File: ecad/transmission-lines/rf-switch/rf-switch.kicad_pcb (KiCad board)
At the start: 2 copper layers, 22.9 x 34.3 mm, 5 parts, among them J1 USB_C_Receptacle_USB2.0, J2 Conn_01x05_Pin, SW1 SW_DIP_x01, U1 ADG918BRM, U2 AP7384-33Y

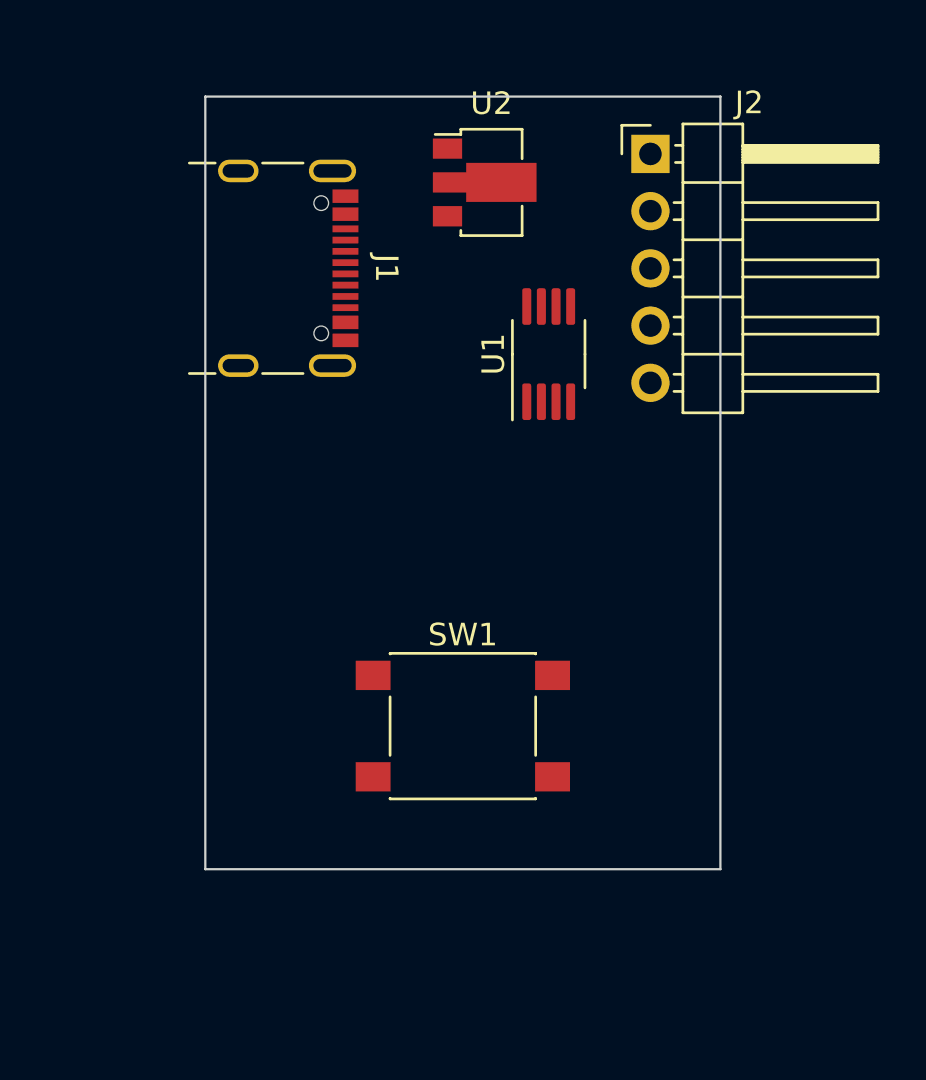
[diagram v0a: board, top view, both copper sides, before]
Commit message: rf-switch: Update
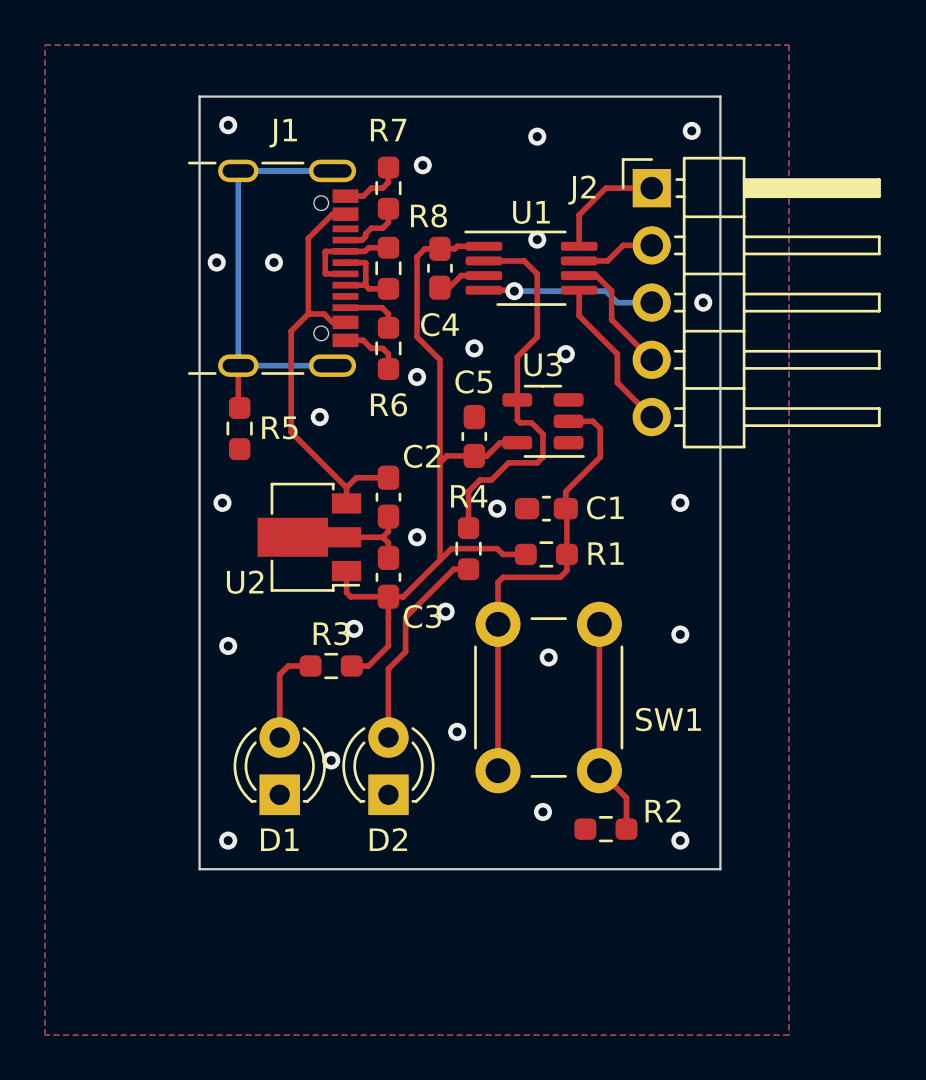
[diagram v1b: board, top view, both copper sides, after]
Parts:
- added C1: 10u, Capacitor_SMD:C_0603_1608Metric_Pad1.08x0.95mm_HandSolder, F.Cu at (140.9, 91.9)
- added C2: C, Capacitor_SMD:C_0603_1608Metric_Pad1.08x0.95mm_HandSolder, F.Cu at (133.9, 91.4)
- added C3: C, Capacitor_SMD:C_0603_1608Metric_Pad1.08x0.95mm_HandSolder, F.Cu at (133.9, 95.0)
- added C4: 100n, Capacitor_SMD:C_0603_1608Metric_Pad1.08x0.95mm_HandSolder, F.Cu at (136.1, 81.3)
- added C5: 100n, Capacitor_SMD:C_0603_1608Metric_Pad1.08x0.95mm_HandSolder, F.Cu at (137.7, 88.7)
- added D1: LED, LED_THT:LED_D3.0mm_FlatTop, F.Cu at (129.0, 104.6)
- added D2: LED, LED_THT:LED_D3.0mm_FlatTop, F.Cu at (133.9, 104.6)
- added R1: 1k, Resistor_SMD:R_0603_1608Metric_Pad0.98x0.95mm_HandSolder, F.Cu at (140.9, 94.0)
- added R2: 1k, Resistor_SMD:R_0603_1608Metric_Pad0.98x0.95mm_HandSolder, F.Cu at (143.5, 106.2)
- added R3: R, Resistor_SMD:R_0603_1608Metric_Pad0.98x0.95mm_HandSolder, F.Cu at (131.3, 98.9)
- added R4: R, Resistor_SMD:R_0603_1608Metric_Pad0.98x0.95mm_HandSolder, F.Cu at (137.4, 93.7)
- added R5: R, Resistor_SMD:R_0603_1608Metric_Pad0.98x0.95mm_HandSolder, F.Cu at (127.3, 88.4)
- added R6: 56k, Resistor_SMD:R_0603_1608Metric_Pad0.98x0.95mm_HandSolder, F.Cu at (133.9, 84.8)
- added R7: 56k, Resistor_SMD:R_0603_1608Metric_Pad0.98x0.95mm_HandSolder, F.Cu at (133.9, 77.7)
- added R8: R, Resistor_SMD:R_0603_1608Metric_Pad0.98x0.95mm_HandSolder, F.Cu at (133.9, 81.3)
- added U3: SN74LVC1G14DBV, Package_TO_SOT_SMD:SOT-23-5, F.Cu at (140.7, 88.1)
- SW1: footprint Button_Switch_SMD:SW_SPST_PTS645 -> Button_Switch_THT:SW_PUSH_6mm_H4.3mm
- moved U2 17.8 mm to (130.0, 93.2), turned to 180 degrees
- moved SW1 7.56 mm to (143.2, 97.1), turned to -90 degrees
- moved U1 3.89 mm to (140.2, 81.3), turned to 0 degrees
- moved J2 1.52 mm to (145.5, 77.7)
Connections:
- J1 pad A1: Net-(J1-GND-PadA1) -> GND
- J1 pad A12: Net-(J1-GND-PadA1) -> GND
- J1 pad A4: Net-(J1-VBUS-PadA4) -> VBUS
- J1 pad A5: unconnected-(J1-CC1-PadA5) -> Net-(J1-CC1)
- J1 pad A6: unconnected-(J1-D+-PadA6) -> Net-(J1-D+-PadA6)
- J1 pad A7: unconnected-(J1-D--PadA7) -> Net-(J1-D--PadA7)
- J1 pad A9: Net-(J1-VBUS-PadA4) -> VBUS
- J1 pad B1: Net-(J1-GND-PadA1) -> GND
- J1 pad B12: Net-(J1-GND-PadA1) -> GND
- J1 pad B4: Net-(J1-VBUS-PadA4) -> VBUS
- J1 pad B5: unconnected-(J1-CC2-PadB5) -> Net-(J1-CC2)
- J1 pad B6: unconnected-(J1-D+-PadB6) -> Net-(J1-D+-PadA6)
- J1 pad B7: unconnected-(J1-D--PadB7) -> Net-(J1-D--PadA7)
- J1 pad B9: Net-(J1-VBUS-PadA4) -> VBUS
- J1 pad S1: unconnected-(J1-SHIELD-PadS1) -> Net-(J1-SHIELD)
- J2 pad 1: unconnected-(J2-Pin_1-Pad1) -> Net-(J2-Pin_1)
- J2 pad 2: unconnected-(J2-Pin_2-Pad2) -> GND
- J2 pad 3: unconnected-(J2-Pin_3-Pad3) -> Net-(J2-Pin_3)
- J2 pad 4: unconnected-(J2-Pin_4-Pad4) -> GND
- J2 pad 5: unconnected-(J2-Pin_5-Pad5) -> Net-(J2-Pin_5)
- SW1 pad 1: unconnected-(SW1-Pad1) -> Net-(R2-Pad2)
- SW1 pad 2: unconnected-(SW1-Pad2) -> Net-(C1-Pad1)
- U1 pad 1: unconnected-(U1-VDD-Pad1) -> +3.3V
- U1 pad 2: unconnected-(U1-CTRL-Pad2) -> Ctrl
- U1 pad 3: Net-(U1-GND-Pad3) -> GND
- U1 pad 4: unconnected-(U1-RFC-Pad4) -> Net-(J2-Pin_3)
- U1 pad 5: unconnected-(U1-RF2-Pad5) -> Net-(J2-Pin_5)
- U1 pad 6: Net-(U1-GND-Pad3) -> GND
- U1 pad 7: Net-(U1-GND-Pad3) -> GND
- U1 pad 8: unconnected-(U1-RF1-Pad8) -> Net-(J2-Pin_1)
- U2 pad 1: unconnected-(U2-VO-Pad1) -> +3.3V
- U2 pad 2: unconnected-(U2-GND-Pad2) -> GND
- U2 pad 3: unconnected-(U2-VI-Pad3) -> VBUS
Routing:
- net +3.3V: track 0.00 -> 35.0 mm
- net GND: track 0.00 -> 20.6 mm, vias 0 -> 26
- net Net-(C1-Pad1): track 0.00 -> 20.1 mm
- net VBUS: track 0.00 -> 19.0 mm
- net Net-(J1-SHIELD): track 0.00 -> 18.9 mm
- net Ctrl: track 0.00 -> 17.4 mm
- net Net-(R2-Pad2): track 0.00 -> 9.59 mm
- net Net-(D2-A): track 0.00 -> 9.33 mm
- net Net-(J2-Pin_3): track 0.00 -> 7.67 mm, vias 0 -> 1
- net Net-(J2-Pin_5): track 0.00 -> 6.96 mm
- net Net-(J2-Pin_1): track 0.00 -> 5.11 mm
- net Net-(J1-D--PadA7): track 0.00 -> 4.75 mm
- net Net-(D1-A): track 0.00 -> 4.33 mm
- net Net-(J1-D+-PadA6): track 0.00 -> 3.87 mm
- net Net-(J1-CC1): track 0.00 -> 2.91 mm
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- added copper zone on B.Cu, net GND
- added copper zone on F.Cu, net GND
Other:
- board size 22.9 x 34.3 mm -> 23.1 x 34.3 mm
